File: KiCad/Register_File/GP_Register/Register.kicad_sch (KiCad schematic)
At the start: 63 parts, among them J1 Conn_01x02_Pin, J2 Conn_01x02_Pin, J3 Conn_01x02_Pin, J4 Conn_01x08_Pin, J5 Conn_01x08_Pin, J6 Conn_01x04_Pin, J7 Conn_01x04_Pin, J8 Conn_01x04_Pin, J9 Conn_01x04_Pin, SW2 SW_SPDT, U1 74LS173, U2 74LS173, U3 74LS245, U4 74LS173, U5 74LS173, U6 74LS245, U7 74LS245, U8 74LS245

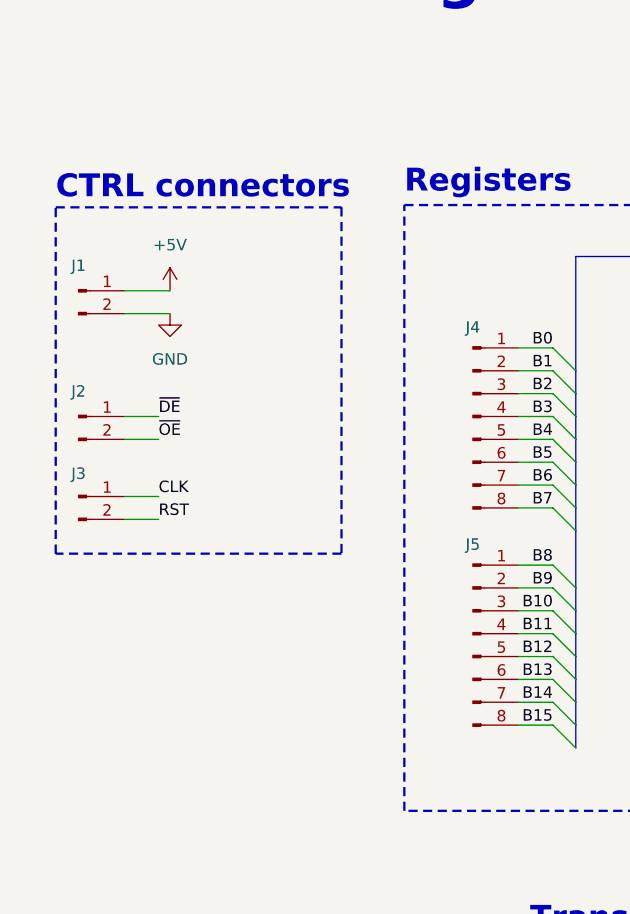
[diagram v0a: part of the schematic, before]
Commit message: added more boards, added pcb standarts
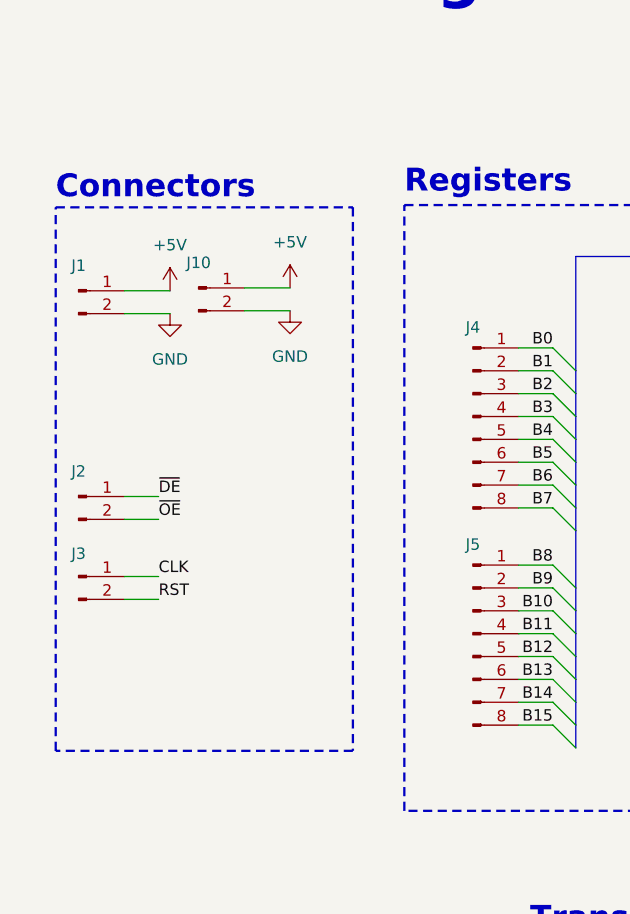
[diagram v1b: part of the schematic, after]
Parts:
- added J10: Conn_01x02_Pin, elad_jst:JST_XH_S2B-XH-A-1_1x02_P2.50mm_Horizontal_fixed, symbol Connector:Conn_01x02_Pin
- C1, C2, C3, C4, C5, C7, C8, C9: footprint Capacitor_THT:C_Disc_D3.8mm_W2.6mm_P2.50mm -> Capacitor_SMD:C_1206_3216Metric_Pad1.33x1.80mm_HandSolder
- J1, J2, J3: footprint Connector_JST:JST_XH_S2B-XH-A_1x02_P2.50mm_Horizontal -> elad_jst:JST_XH_S2B-XH-A-1_1x02_P2.50mm_Horizontal_fixed
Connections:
- net +5V: now also J10.1 (Pin_1)
- net GND: now also J10.2 (Pin_2)
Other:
- note added: "Connectors"
- note removed: "CTRL connectors"
- moved on the sheet: J2, J3
